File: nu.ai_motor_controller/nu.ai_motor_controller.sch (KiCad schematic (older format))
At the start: 17 parts

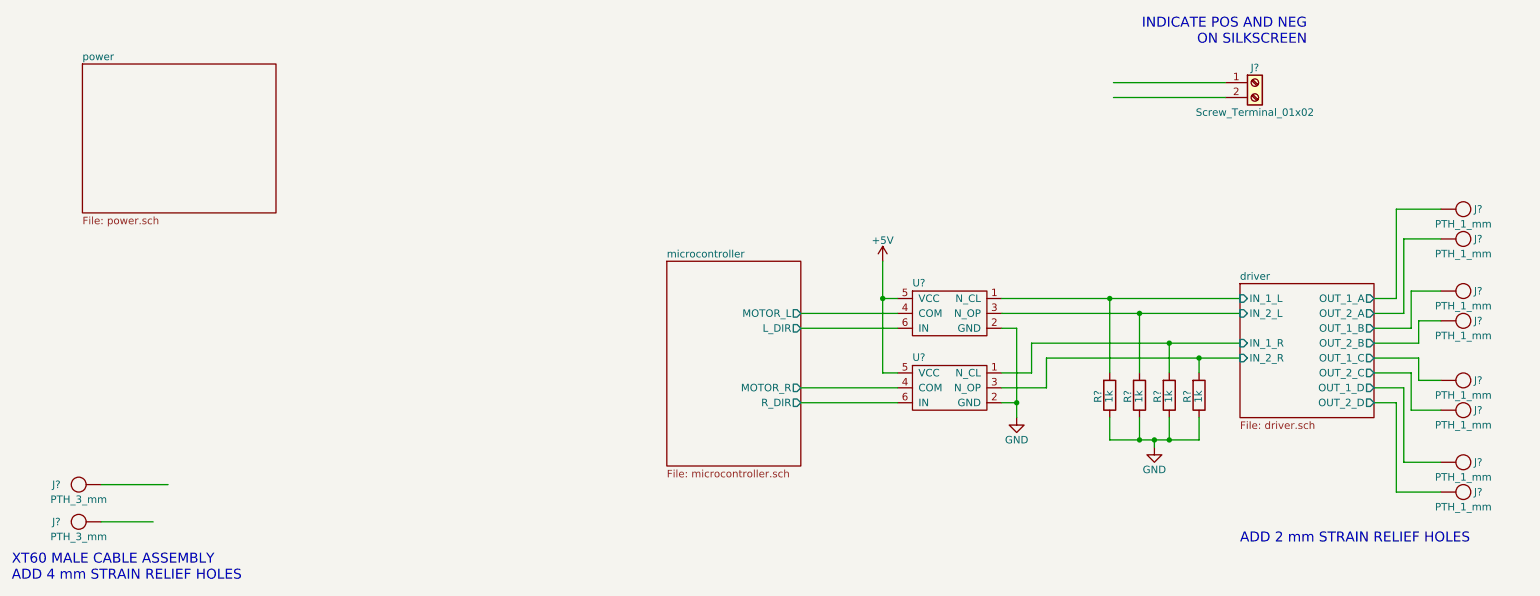
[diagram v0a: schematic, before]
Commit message: automated commit
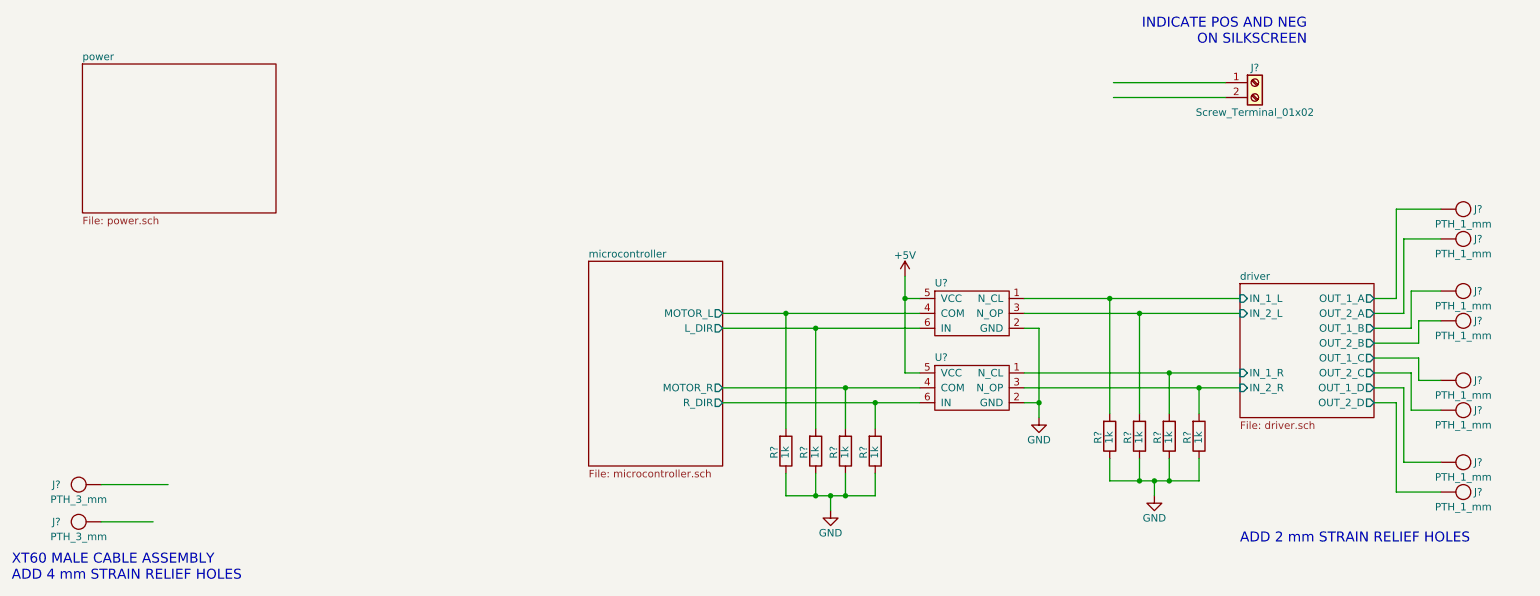
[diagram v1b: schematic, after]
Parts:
- added R? (x4): RC0603JR-071KL, 0603, symbol custom:RC0603JR-071KL
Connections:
- wire segments 65 -> 78
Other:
- moved on the sheet: R?, U?
